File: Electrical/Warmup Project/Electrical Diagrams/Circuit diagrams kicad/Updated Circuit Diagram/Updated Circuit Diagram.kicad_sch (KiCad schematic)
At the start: 24 parts, among them M1 Motor_DC, M2 Motor_DC, M3 Motor_DC, U3 MCP2562-H_SN, U4 Teensy4.1, U5 MCP2562-H_SN, U7 MCP2562-H_SN

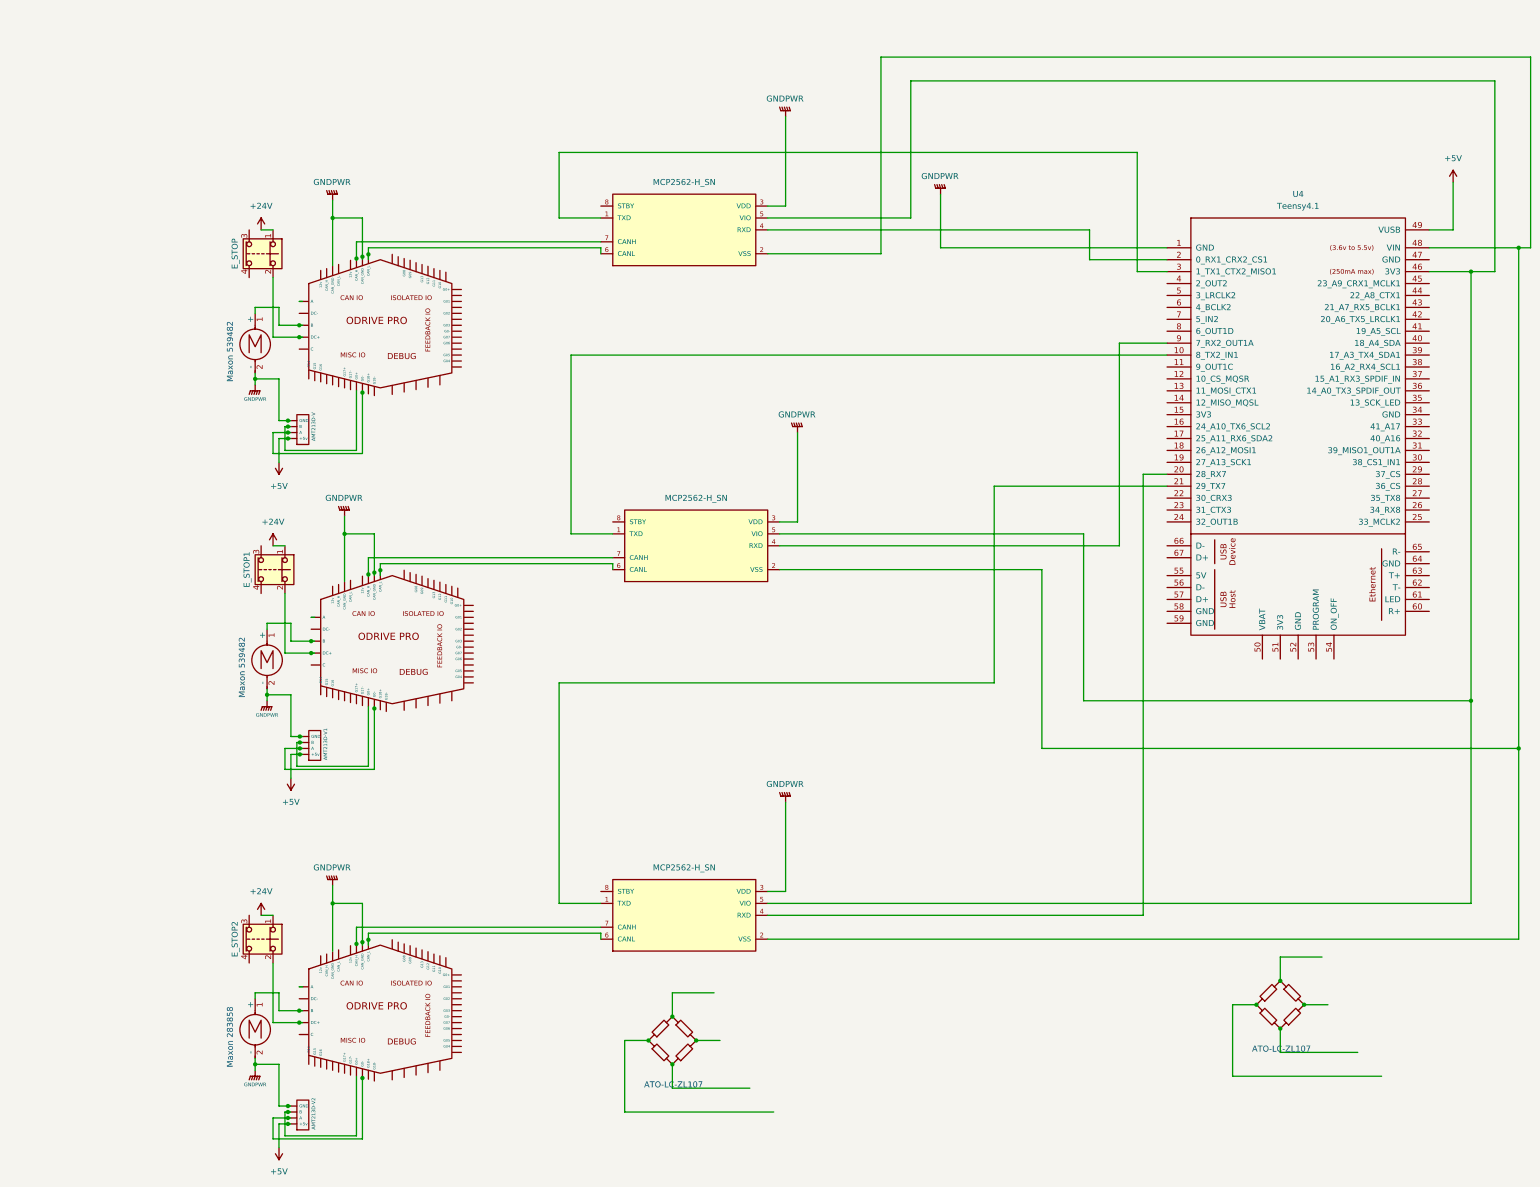
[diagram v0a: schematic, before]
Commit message: Updated Circuit Diagrams
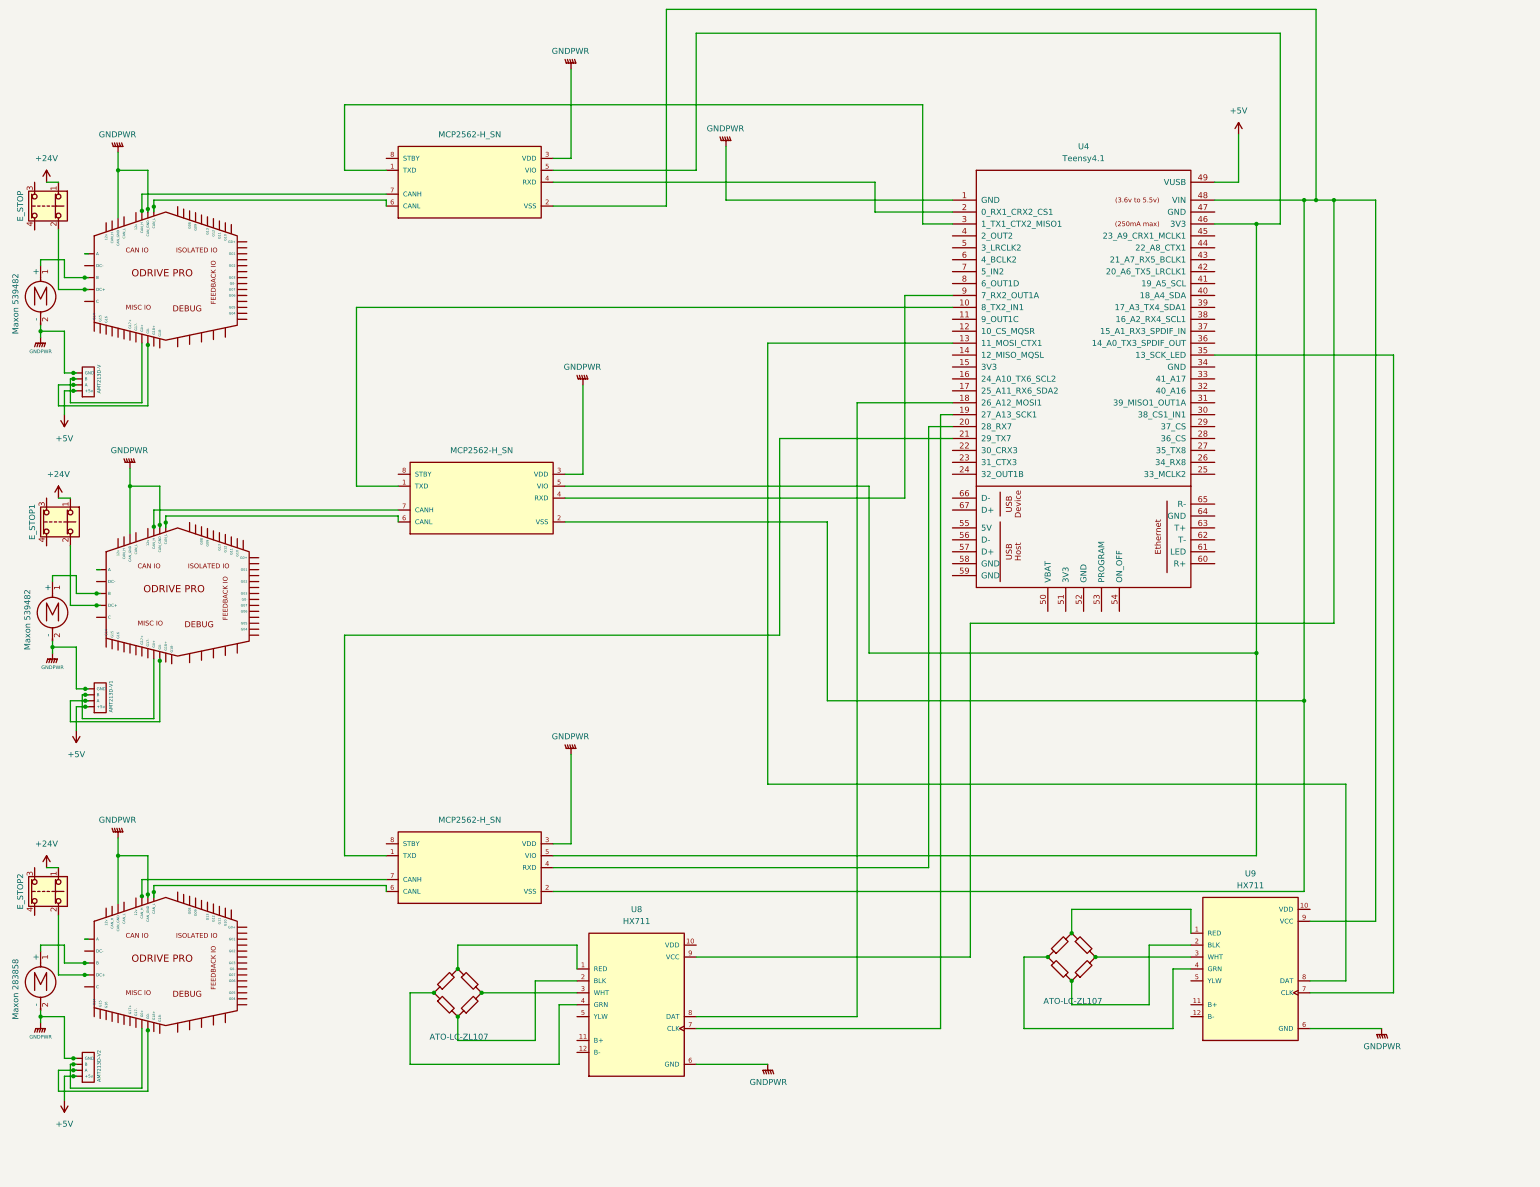
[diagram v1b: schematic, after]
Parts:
- removed R10, R11, R12, R9: R_45deg, symbol Device:R_45deg
- added R2, R3, R4, R5: R_45deg, symbol Device:R_45deg
- added U8, U9: HX711, SEN-13879:SPARKFUN_SEN-13879, symbol SEN-13879:SEN-13879
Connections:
- net GNDPWR: now also U8.6 (GND), U9.6 (GND)
- net at R1.1, R6.1: now also U8.4 (GRN)
- net at R6.2, R8.1: now also U8.2 (BLK)
- net at R1.2, R7.1: now also U8.1 (RED)
- net at R7.2, R8.2: now also U8.3 (WHT)
- net at U3.2 (VSS), U4.48 (VIN), U5.2 (VSS)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: now also U8.9 (VCC), U9.9 (VCC)
- net at U4.13 (11_MOSI_CTX1): now also U9.8 (DAT)
- net at U4.18 (26_A12_MOSI1): now also U8.8 (DAT)
- net at U4.19 (27_A13_SCK1): now also U8.7 (CLK)
- net at U4.35 (13_SCK_LED): now also U9.7 (CLK)
- new net: AMT213D-V2. (GND), U6. (x2)
- new net: R3.2, R5.1, U9.2 (BLK)
- new net: R4.2, R5.2, U9.3 (WHT)
- new net: R2.1, R3.1, U9.4 (GRN)
- new net: R2.2, R4.1, U9.1 (RED)
- new net: AMT213D-V1. (GND), U2. (x2)
- new net: AMT213D-V. (GND), U1. (x2)
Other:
- moved on the sheet: AMT213D-V, AMT213D-V1, AMT213D-V2, E_STOP, E_STOP1, E_STOP2, U4
